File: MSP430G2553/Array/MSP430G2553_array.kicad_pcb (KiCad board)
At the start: 2 copper layers, 51 x 76 mm, 58 parts, among them J1 Power, J2 Programmer, J3 Conn_01x06_Female, J4 Conn_01x08_Female, SW1 SW_Push, U1 MSP430G2553IPW20, Y1 Crystal_GND24

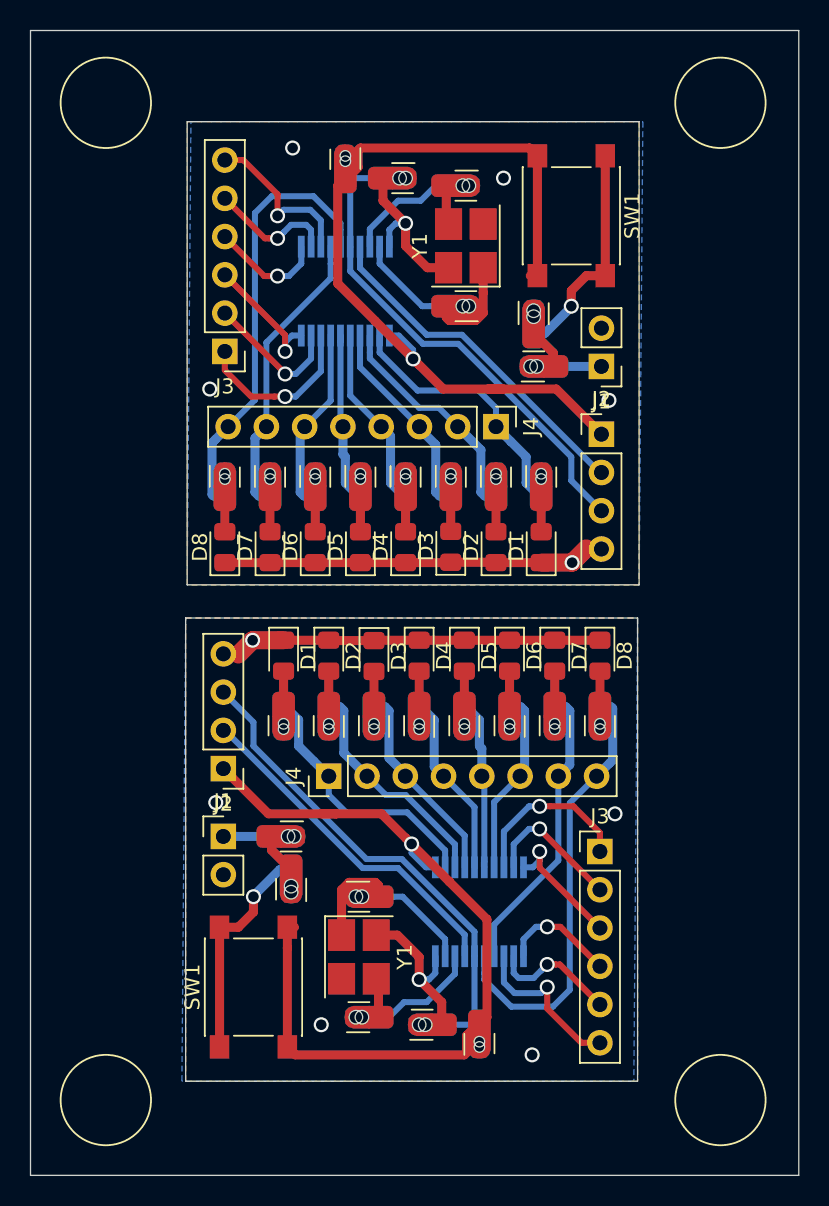
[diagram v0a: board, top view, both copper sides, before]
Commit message: new msp board and array.
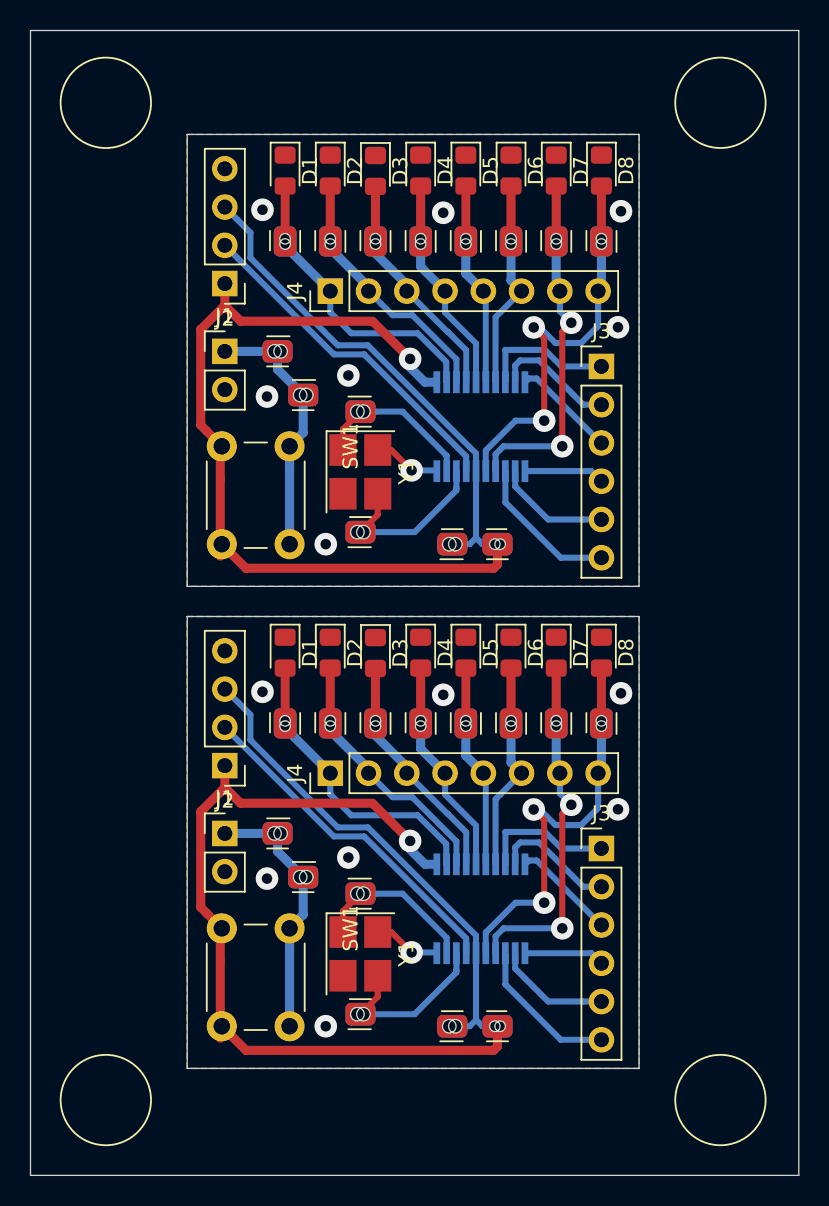
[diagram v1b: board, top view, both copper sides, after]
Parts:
- removed the U1 at (110.9, 56.3)
- removed the U1 at (119.8, 97.5)
- added U1: MSP430G2553IPW20, Package_SO:TSSOP-20_4.4x6.5mm_P0.65mm, B.Cu at (119.9, 97.3)
- added U1: MSP430G2553IPW20, Package_SO:TSSOP-20_4.4x6.5mm_P0.65mm, B.Cu at (119.9, 65.3)
- C1 (x2), C2 (x2), C3 (x2), C4 (x2), C5 (x2): footprint thSMD:thsmd_03_l -> thSMD:thsmd_04_l
- R1 (x2), R2 (x2), R3 (x2), R4 (x2), R5 (x2), R6 (x2), R7 (x2), R8 (x2), R9 (x2): footprint thSMD:thsmd_03_s -> thSMD:thsmd_04_s
- SW1 (x2): footprint Button_Switch_SMD:SW_Push_1P1T_NO_6x6mm_H9.5mm -> Button_Switch_THT:SW_PUSH_6mm
- moved R1 58.5 mm to (121.0, 105.1), turned to 0 degrees
- moved C4 56.4 mm to (118.0, 105.1), turned to 180 degrees
- moved C5 55.4 mm to (111.9, 104.3), turned to 180 degrees
- moved SW1 50.9 mm to (107.2, 98.6)
- moved Y1 47.5 mm to (111.9, 100.3), turned to 270 degrees
- moved J3 41.4 mm to (127.9, 93.3), turned to 0 degrees
- moved C2 40.4 mm to (108.1, 95.2), turned to 0 degrees
- moved J1 39.8 mm to (102.9, 92.3), turned to 0 degrees
- moved C1 39.6 mm to (111.9, 96.3), turned to 180 degrees
- moved SW1 36.0 mm to (107.2, 66.6), turned to 270 degrees
- moved C3 35.4 mm to (106.4, 92.3), turned to 0 degrees
- moved J2 33.3 mm to (102.9, 87.8), turned to 180 degrees
- moved R1 33.2 mm to (121.0, 73.1), turned to 0 degrees
- moved C2 32.8 mm to (108.1, 63.2), turned to 0 degrees
- moved C3 32.2 mm to (106.4, 60.3)
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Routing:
- net GND: track 76.2 -> 9.01 mm, vias 12 -> 16
- net P1.7: track 58.4 -> 46.9 mm, vias 0 -> 4
- net Net-(C2-Pad1): track 41.7 -> 34.8 mm, vias 2 -> 0
- net Net-(C1-Pad1): track 13.0 -> 6.05 mm
- net P2.0: track 22.8 -> 18.0 mm, vias 2 -> 0
- net P2.3: track 15.3 -> 10.7 mm, vias 2 -> 0
- net P1.5: track 24.7 -> 20.7 mm
- net P1.1: track 30.6 -> 27.2 mm
- net P1.2: track 27.2 -> 23.7 mm
- net P2.2: track 17.2 -> 13.9 mm, vias 2 -> 0
- net P1.4: track 22.6 -> 19.8 mm
- net P1.3: track 24.5 -> 21.7 mm
- net Net-(C5-Pad1): track 14.9 -> 17.6 mm
- net Net-(D3-Pad2): track 4.70 -> 7.30 mm
- net Net-(D8-Pad2): track 4.75 -> 7.35 mm
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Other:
- outline, holes or cut-outs redrawn
